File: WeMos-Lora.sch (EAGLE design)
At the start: 27 parts, among them P1 PADNORMAL, P2 PADNORMAL, P3 PADNORMAL, P4 PADNORMAL, U1 24AA02E64T

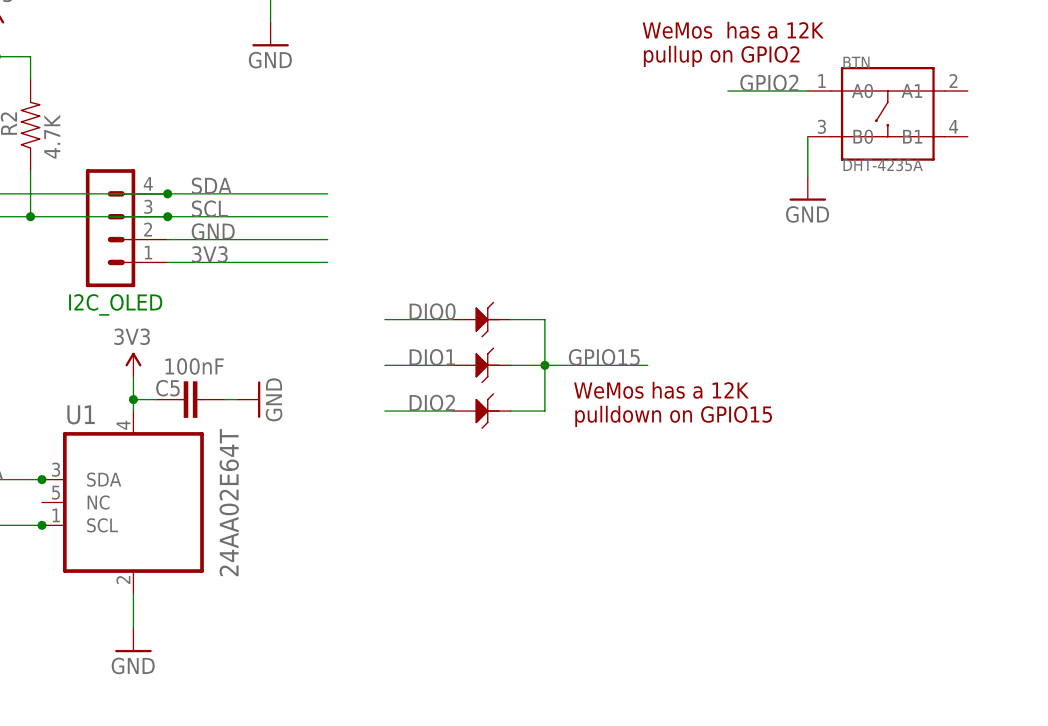
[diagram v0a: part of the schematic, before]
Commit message: Bump to v1.3
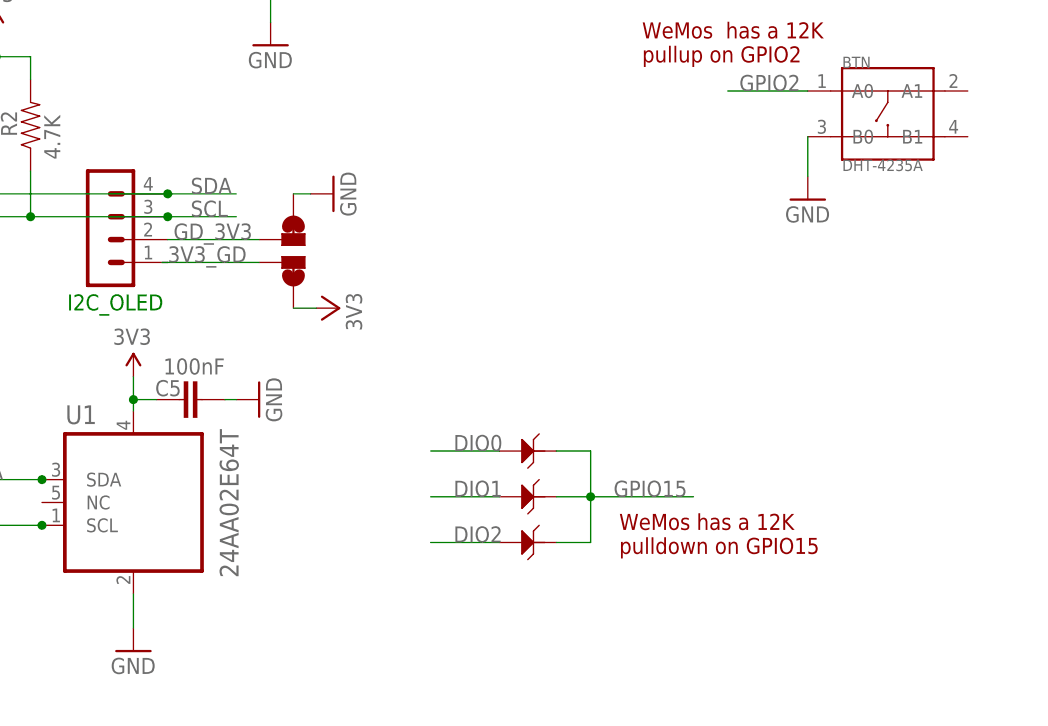
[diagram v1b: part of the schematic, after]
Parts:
- added U$2: PAD-JUMPER-SWAPSWAP, _c2h:PAD-JUMPER-SWAPSWAP
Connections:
- new net 3V3_GD: I2C_OLED.1, U$2.3
- new net GD_3V3: I2C_OLED.2, U$2.2
- net 3V3: now also U$2.4; no longer I2C_OLED.1
- net GND: now also U$2.1; no longer I2C_OLED.2
